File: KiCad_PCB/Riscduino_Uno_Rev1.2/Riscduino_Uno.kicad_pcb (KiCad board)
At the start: 2 copper layers, 70.6 x 53.7 mm, 95 parts, among them J1 Conn_01x06_Pin, J10 Conn_01x10_Pin, J11 USB_B_Micro, J2 Conn_01x08_Pin, J3 Conn_01x01, J4 Conn_02x04_Odd_Even, J5 ISP, J6 Conn_01x01, J7 Conn_01x01, J8 Conn_01x01, J9 Conn_01x08_Pin, SW1 4Pin Round Button SPST Straig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, U1 MAX1232ESA+T, U2 W25Q32JVSS, U3 23LC1024-I/P, U4 W25Q32JVSS, U5 Riscduino, U6 LM1117MP-3.3, U7 LM1117S-ADJ, U8 CH340C, X1 ASE-10.000MHZ-LC-T

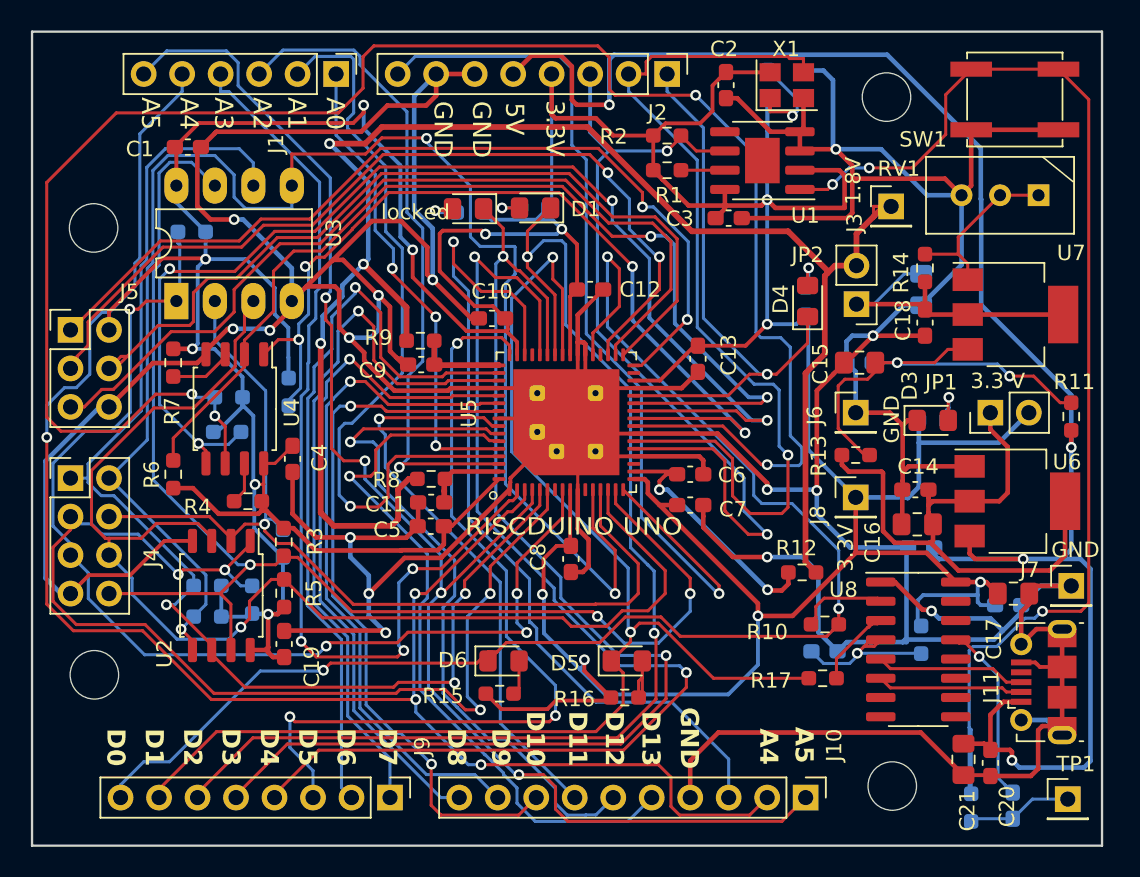
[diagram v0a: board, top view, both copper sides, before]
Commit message: Rev Uno 1.2 update
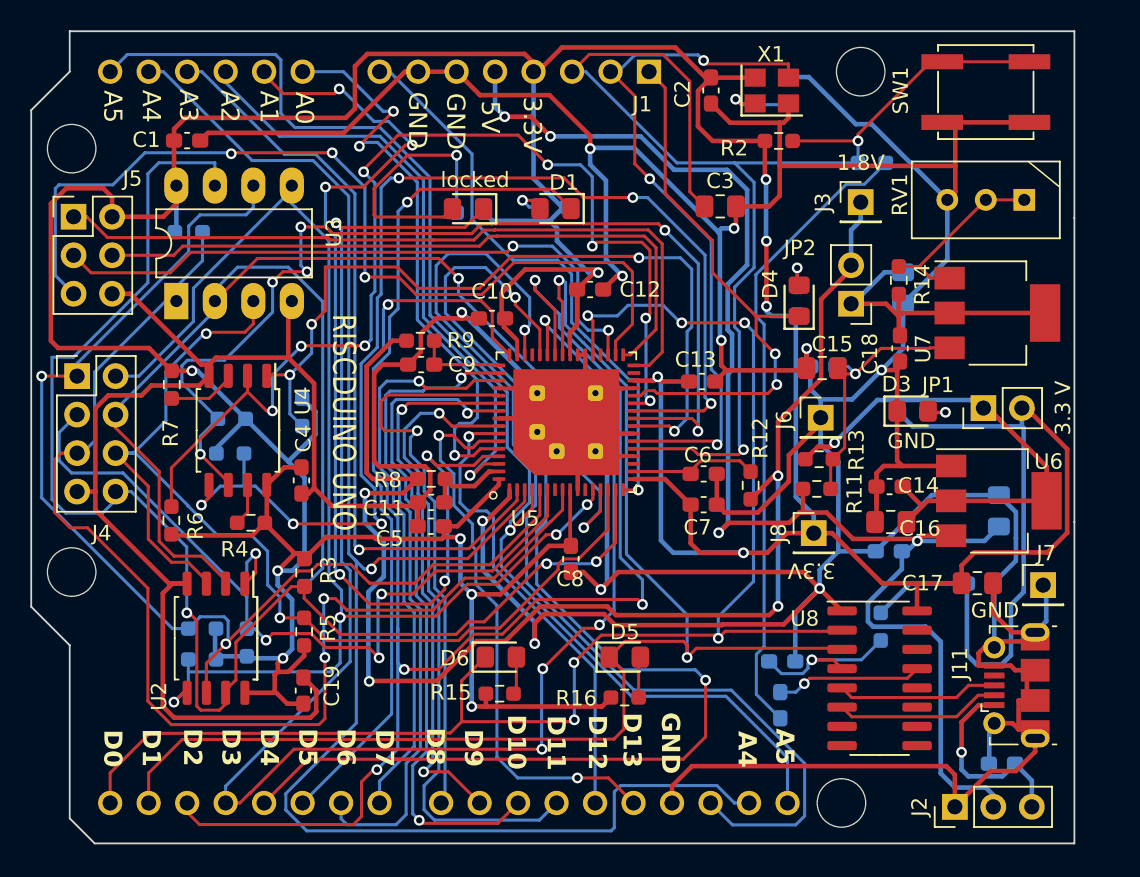
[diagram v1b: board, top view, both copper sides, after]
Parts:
- removed H1, H2, H3, H4: MountingHole, MountingHole:MountingHole_3.2mm_M3
- removed J10: Conn_01x10_Pin, Connector_PinHeader_2.54mm:PinHeader_1x10_P2.54mm_Vertical
- removed J9: Conn_01x08_Pin, Connector_PinHeader_2.54mm:PinHeader_1x08_P2.54mm_Vertical
- removed R1: 10K, Resistor_SMD:R_0603_1608Metric_Pad0.98x0.95mm_HandSolder
- removed R10, R17: 0E, Resistor_SMD:R_0603_1608Metric_Pad0.98x0.95mm_HandSolder
- removed R18: DNI, Resistor_SMD:R_0603_1608Metric_Pad0.98x0.95mm_HandSolder
- removed TP1: TestPoint, Connector_PinHeader_2.54mm:PinHeader_1x01_P2.54mm_Vertical
- removed U1: MAX1232ESA+T, Package_SO:SOIC-8-1EP_3.9x4.9mm_P1.27mm_EP2.29x3mm
- C20, C21: moved to B.Cu
- C3: value 0.1uf -> 10uF; footprint Capacitor_SMD:C_0603_1608Metric_Pad1.08x0.95mm_HandSolder -> Capacitor_SMD:C_0805_2012Metric_Pad1.18x1.45mm_HandSolder
- D1, D3, D4, D5, locked: footprint LED_SMD:LED_0805_2012Metric_Pad1.15x1.40mm_HandSolder -> Riscduino:LED_0805_2012Metric_Pad1.15x1.40mm_HandSolder
- D6: footprint LED_SMD:LED_0805_2012Metric_Pad1.15x1.40mm_HandSolder -> Riscduino.Library:LED_0805_2012Metric_Pad1.15x1.40mm_HandSolder
- J1: value Conn_01x06_Pin -> Conn_01x32_Pin; footprint Connector_PinHeader_2.54mm:PinHeader_1x06_P2.54mm_Vertical -> Riscduino.Library:Arduino_UNO_R3_WithMountingHoles
- J2: value Conn_01x08_Pin -> Conn_01x03_Pin; footprint Connector_PinHeader_2.54mm:PinHeader_1x08_P2.54mm_Vertical -> Connector_PinHeader_2.54mm:PinHeader_1x03_P2.54mm_Vertical
- RV1: footprint Potentiometer_THT:Potentiometer_Bourns_3296W_Vertical -> Riscduino.Library:Potentiometer_Bourns_3296W_Vertical
- X1: footprint Crystal:Crystal_SMD_Abracon_ABM8G-4Pin_3.2x2.5mm -> Riscduino:Crystal_SMD_Abracon_ABM8G-4Pin_3.2x2.5mm
- moved J2 52.0 mm to (130.2, 100.7), turned to 90 degrees
- moved R32 43.0 mm to (124.8, 58.2), turned to 180 degrees
- moved J1 20.7 mm to (110.1, 52.2), turned to 0 degrees
- moved R11 17.5 mm to (121.1, 79.7), turned to 0 degrees
- moved C26 16.7 mm to (118.7, 94.0)
- moved C21 16.6 mm to (133.1, 81.2), turned to 90 degrees
- moved J5 7.47 mm to (72.1, 61.7)
- moved R2 7.37 mm to (118.6, 56.7)
- moved J4 6.74 mm to (72.3, 72.3)
- moved R12 6.67 mm to (116.8, 79.5), turned to -90 degrees
- moved J8 3.64 mm to (120.9, 82.6)
- moved C19 3.33 mm to (87.2, 93.0)
- moved U8 3.19 mm to (125.3, 92.2)
- moved R6 3.05 mm to (78.5, 81.8)
- moved C27 2.87 mm to (118.8, 91.1)
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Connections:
- C20 pad 1: +5V -> +5VP
- C3 pad 1: +3.3V -> ~{RST}
- J1 pad 1: ardunio_a0 -> gpio
- J1 pad 2: ardunio_a1 -> xclk
- J1 pad 3: ardunio_a2 -> ~{RST}
- J1 pad 4: ardunio_a3 -> +3.3V
- J1 pad 5: ardunio_a4 -> +5V
- J1 pad 6: ardunio_a5 -> GND
- J11 pad 1: +5V -> +5VP
- J2 pad 1: gpio -> GND
- J2 pad 2: xclk -> +5V
- J2 pad 3: ~{RST} -> +5VP
- R32 pad 2: ~{PB_RST} -> ~{RST}
- SW1 pad 2: ~{PB_RST} -> ~{RST}
- U5 pad 24: CARAVEL_FLASH_SCK -> CARAVEL_FLASH_SSN
- U5 pad 25: CARAVEL_FLASH_SSN -> CARAVEL_FLASH_SCK
- U8 pad 2: Net-(U8-TXD) -> ardunio_d0
- U8 pad 3: Net-(U8-RXD) -> ardunio_d1
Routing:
- net ~{PB_RST}: track 80.9 -> 0.00 mm, vias 3 -> 0
- net CARAVEL_FLASH_SCK: track 123.2 -> 68.7 mm, vias 4 -> 6
- net ardunio_d2: track 79.4 -> 117.4 mm, vias 2 -> 5
- net Net-(C26-Pad2): track 6.73 -> 42.0 mm
- net ardunio_d3: track 78.4 -> 109.9 mm, vias 2 -> 5
- net USER_FLASH_IO1: track 64.1 -> 94.5 mm, vias 1 -> 2
- net ~{RST}: track 57.4 -> 85.4 mm
- net mprj_io_37: track 60.5 -> 37.5 mm
- net USER_FLASH_IO0: track 105.2 -> 86.0 mm, vias 3 -> 4
- net +5V: track 113.6 -> 94.5 mm
- net ardunio_a1: track 50.2 -> 67.7 mm, vias 1 -> 6
- net +1V8: track 108.8 -> 91.7 mm, vias 3 -> 4
- net ardunio_d12: track 46.5 -> 30.9 mm
- net ISP_SCK: track 57.2 -> 42.3 mm
- net Net-(D2-A): track 2.49 -> 17.4 mm
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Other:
- board size 70.6 x 53.7 mm -> 68.8 x 53.6 mm
- board text added: "J1"

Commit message: Riscduino Uno Rev1.2
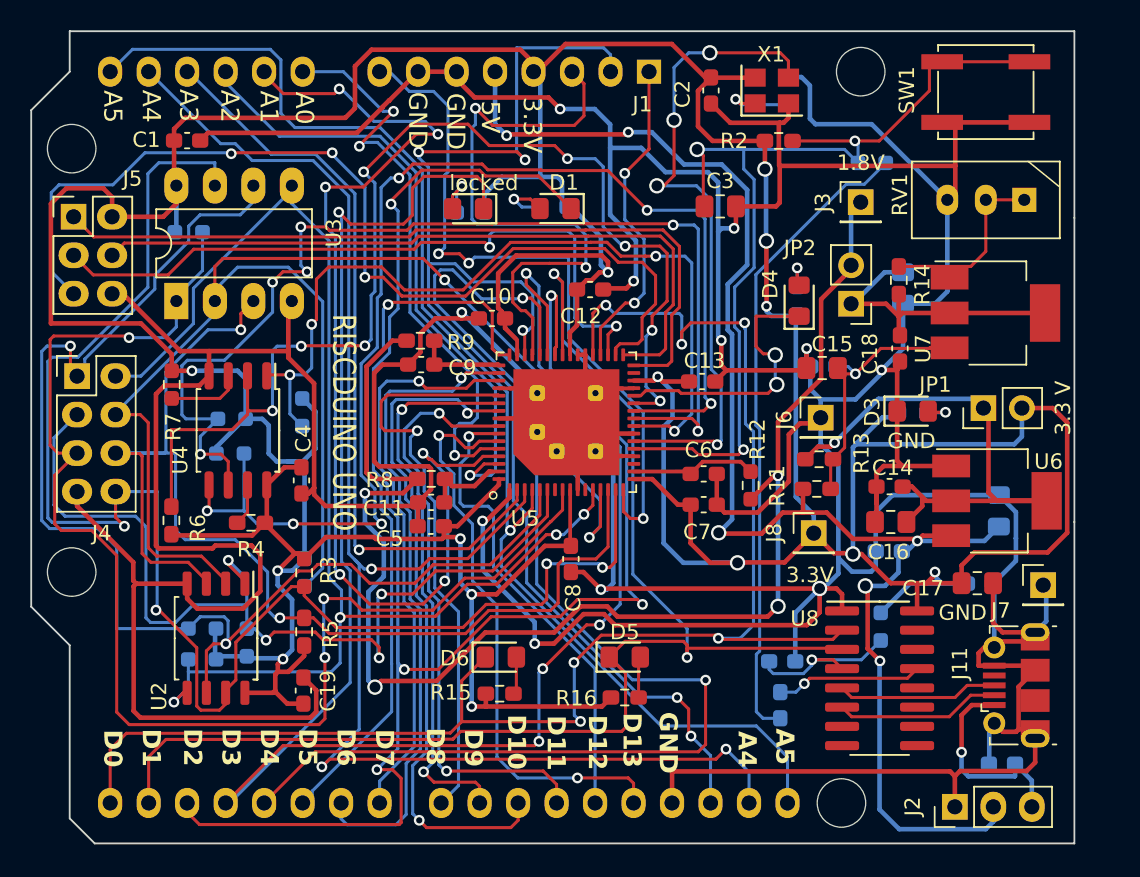
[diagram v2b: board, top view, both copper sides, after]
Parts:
- U2: footprint Package_SO:SOIC-8_5.23x5.23mm_P1.27mm -> Riscduino:SOIC-8_5.23x5.23mm_P1.27mm
- U4: footprint Package_SO:SOIC-8_5.23x5.23mm_P1.27mm -> Riscduino.Library:SOIC-8_5.23x5.23mm_P1.27mm
- U8: footprint Package_SO:SOIC-16_3.9x9.9mm_P1.27mm -> Riscduino:SOIC-16_3.9x9.9mm_P1.27mm
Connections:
- J1 pad 1: gpio -> mprj_io_5_ser_rx
- J1 pad 2: xclk -> mprj_io_12
- J1 pad 3: ~{RST} -> mprj_io_11
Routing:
- net mprj_io_11: track 0.00 -> 40.0 mm, vias 0 -> 2
- net GND: track 466.9 -> 496.1 mm
- net ~{RST}: track 85.4 -> 63.0 mm, vias 2 -> 3
- net mprj_io_5_ser_rx: track 0.00 -> 21.4 mm, vias 0 -> 2
- net gpio: track 36.9 -> 18.2 mm
- net mprj_io_12: track 69.3 -> 87.0 mm, vias 1 -> 5
- net Net-(D2-A): track 17.4 -> 3.61 mm
- net ardunio_d3: track 109.9 -> 121.2 mm
- net mprj_io_37: track 37.5 -> 46.0 mm, vias 1 -> 3
- net USER_SRAM_SSN: track 79.2 -> 87.3 mm, vias 2 -> 3
- net ardunio_a4: track 107.6 -> 100.8 mm, vias 1 -> 3
- net USER_FLASH_IO3: track 94.4 -> 101.2 mm, vias 3 -> 4
- net USER_FLASH_SSN: track 56.2 -> 62.9 mm
- net USER_FLASH_IO2: track 73.1 -> 79.7 mm
- net CARAVEL_FLASH_IO1: track 71.5 -> 77.9 mm
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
